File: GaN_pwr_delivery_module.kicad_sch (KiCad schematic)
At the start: 42 parts, among them J1 dcConn, J2 gateConn, J3 drainConn, Q1 AONS66920, U1 LDO40LPURY, U2 LM2662MX_NOPB, U3 LT4256-1CS8, U4 LM324

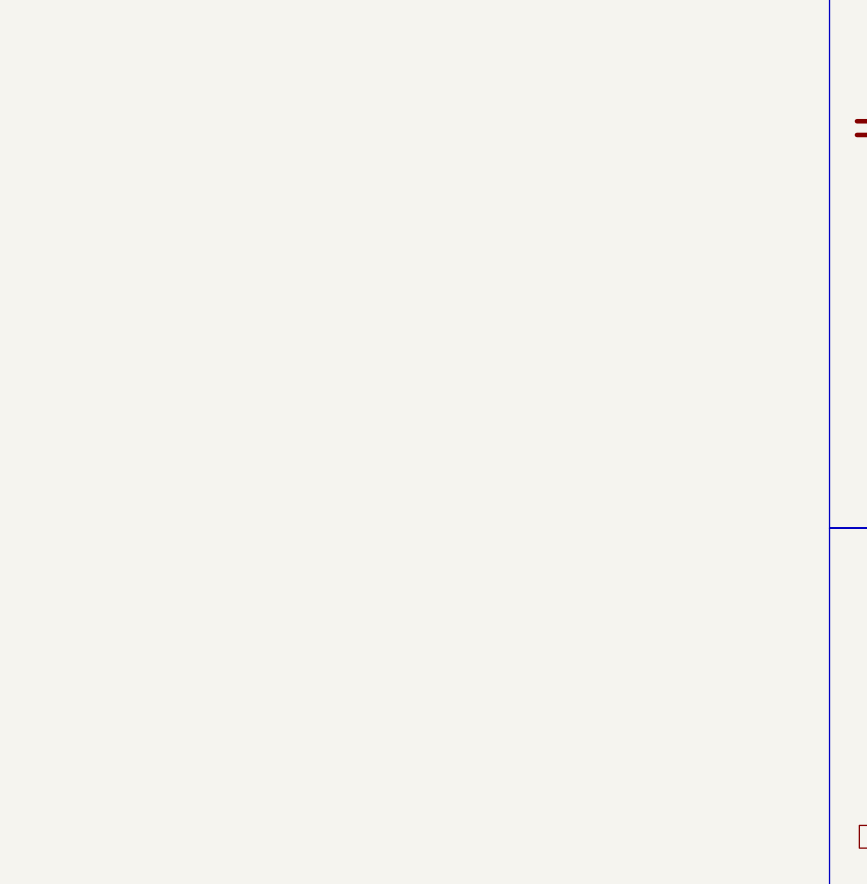
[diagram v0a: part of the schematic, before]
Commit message: POC
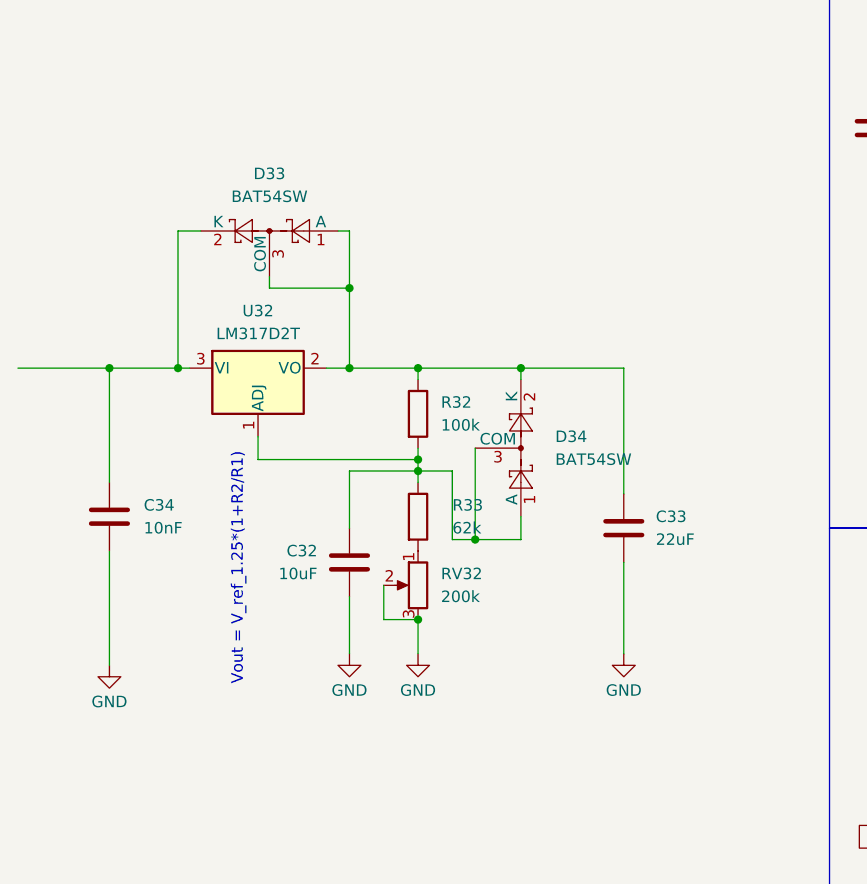
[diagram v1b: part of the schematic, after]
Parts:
- added C32: 10uF, Capacitor_SMD:CP_Elec_6.3x9.9, symbol Device:C
- added C33: 22uF, Capacitor_SMD:CP_Elec_6.3x9.9, symbol Device:C
- added C34: 10nF, Capacitor_SMD:C_0805_2012Metric_Pad1.18x1.45mm_HandSolder, symbol Device:C
- added D33, D34: BAT54SW, Package_TO_SOT_SMD:SOT-323_SC-70, symbol Diode:BAT54SW
- added R32: 100k, Resistor_SMD:R_0805_2012Metric, symbol Device:R
- added R33: 62k, Resistor_SMD:R_0805_2012Metric, symbol Device:R
- added RV32: 200k, Potentiometer_THT:Potentiometer_Bourns_3296W_Vertical, symbol Device:R_Potentiometer
- added U32: LM317D2T, LM317D2T:VREG_L7805ACD2T, symbol Regulator_Linear:LM317L_SOT-89
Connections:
- net GND: now also C32.2, C33.2, C34.2, RV32.2, RV32.3
- new net: C33.1, D33.1 (A), D33.3 (COM), D34.2 (K), R32.1, U32.2 (VO)
- new net: C34.1, D33.2 (K), U32.3 (VI)
- new net: C32.1, D34.1 (A), D34.3 (COM), R32.2, R33.1, U32.1 (ADJ)
- new net: R33.2, RV32.1
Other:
- note added: "Vout = V_ref_1.25*(1+R2/R1)"
